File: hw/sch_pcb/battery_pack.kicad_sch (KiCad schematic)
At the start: 3 parts, among them J1 HEADER_2x03_PARALLEL

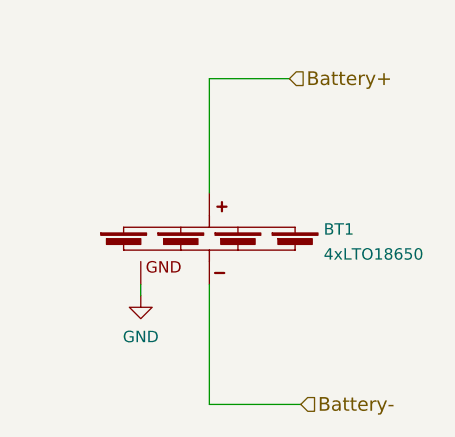
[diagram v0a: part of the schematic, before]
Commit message: Edit PCB
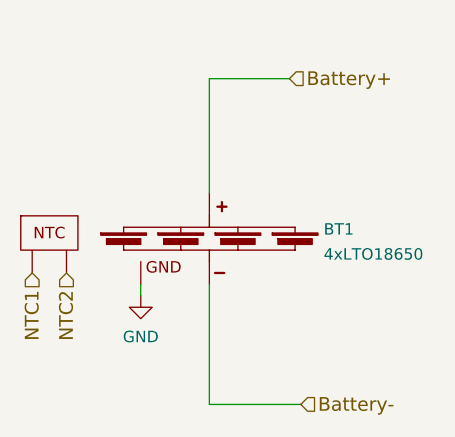
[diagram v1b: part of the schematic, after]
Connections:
- new net NTC1: BT1.5
- new net NTC2: BT1.6
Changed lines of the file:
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@@
     (effects (font (size 1.524 1.524)) (justify left))
+  )
+  (hierarchical_label "NTC1" (shape input) (at 101.6 100.965 270)
+    (effects (font (size 1.524 1.524)) (justify right))
+  )
+  (hierarchical_label "NTC2" (shape input) (at 105.41 100.965 270)
+    (effects (font (size 1.524 1.524)) (justify right))
   )
   (hierarchical_label "Battery-" (shape input) (at 131.445 115.57 0)
@@
     (pin "2")
     (pin "3")
+    (pin "5")
+    (pin "6")
   )
   (symbol (lib_id "MLAB_HEADER:HEADER_2x03_PARALLEL") (at 228.6 94.615 0) (unit 1)

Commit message: Edit UST ID
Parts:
- F1: UST_ID (none) -> 5c70984512875079b91f88d3
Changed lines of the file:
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@@
+      (effects (font (size 1.27 1.27)) hide)
+    )
+    (property "UST_ID" "5c70984512875079b91f88d3" (id 4) (at 212.725 94.615 0)
       (effects (font (size 1.27 1.27)) hide)
     )
